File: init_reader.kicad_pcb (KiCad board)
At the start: 2 copper layers, 95 x 60 mm, 0 parts

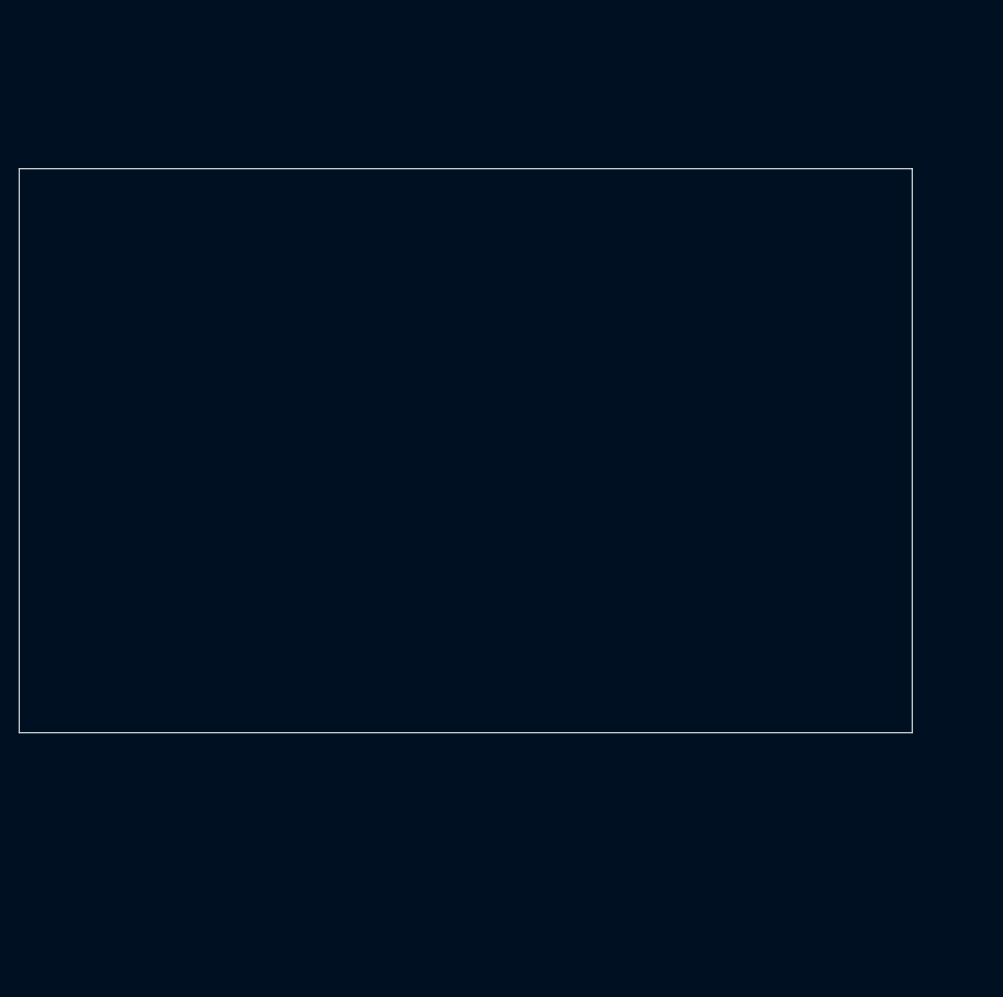
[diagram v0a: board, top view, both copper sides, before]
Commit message: update schematics
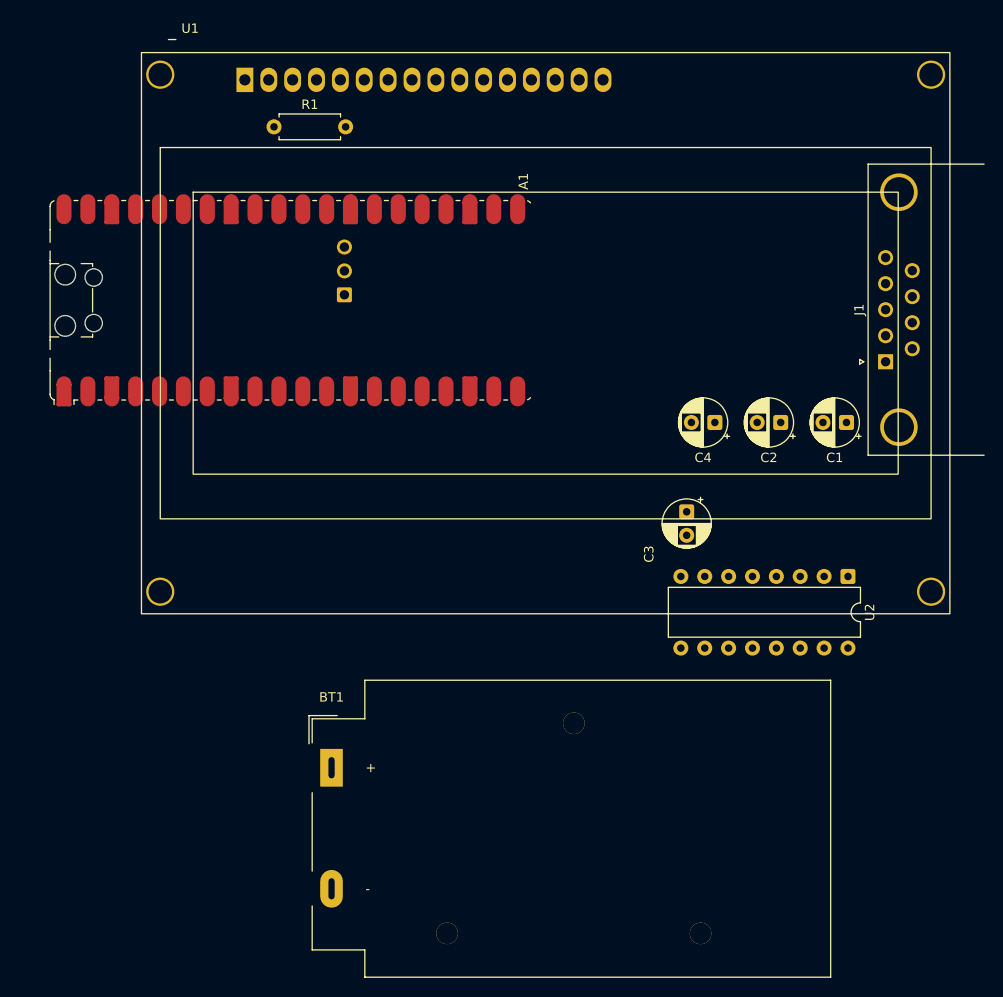
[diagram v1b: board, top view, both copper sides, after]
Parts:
- added A1: RaspberryPi_Pico_W, Module:RaspberryPi_Pico_W_SMD_HandSolder, F.Cu at (123.9, 74.0)
- added BT1: Battery, Battery:BatteryHolder_MPD_BA9VPC_1xPP3, F.Cu at (128.2, 123.7)
- added C1: 10uF, Capacitor_THT:CP_Radial_D5.0mm_P2.50mm, F.Cu at (183.0, 87.0)
- added C2: 10uF, Capacitor_THT:CP_Radial_D5.0mm_P2.50mm, F.Cu at (176.0, 87.0)
- added C3: 10uF, Capacitor_THT:CP_Radial_D5.0mm_P2.50mm, F.Cu at (166.0, 96.5)
- added C4: 10uF, Capacitor_THT:CP_Radial_D5.0mm_P2.50mm, F.Cu at (169.0, 87.0)
- added J1: DE9_Pins, Connector_Dsub:DSUB-9_Pins_Horizontal_P2.77x2.84mm_EdgePinOffset7.70mm_Housed_MountingHolesOffset9.12mm, F.Cu at (187.2, 80.5)
- added R1: R, Resistor_THT:R_Axial_DIN0207_L6.3mm_D2.5mm_P7.62mm_Horizontal, F.Cu at (122.1, 55.5)
- added U1: LCD_16x4, 0_moje:AC-164A, F.Cu at (151.0, 77.5)
- added U2: MAX232, Package_DIP:DIP-16_W7.62mm, F.Cu at (183.2, 103.4)
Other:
- board outline removed
